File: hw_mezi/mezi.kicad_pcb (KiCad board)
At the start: 2 copper layers, 49.7 x 62.2 mm, 32 parts, among them J1 Conn_2Rows-05Pins, SW1 SW_DPST_x2, T1 Tab, T53,086 Tab, U1 PY32F002AF15P6TU

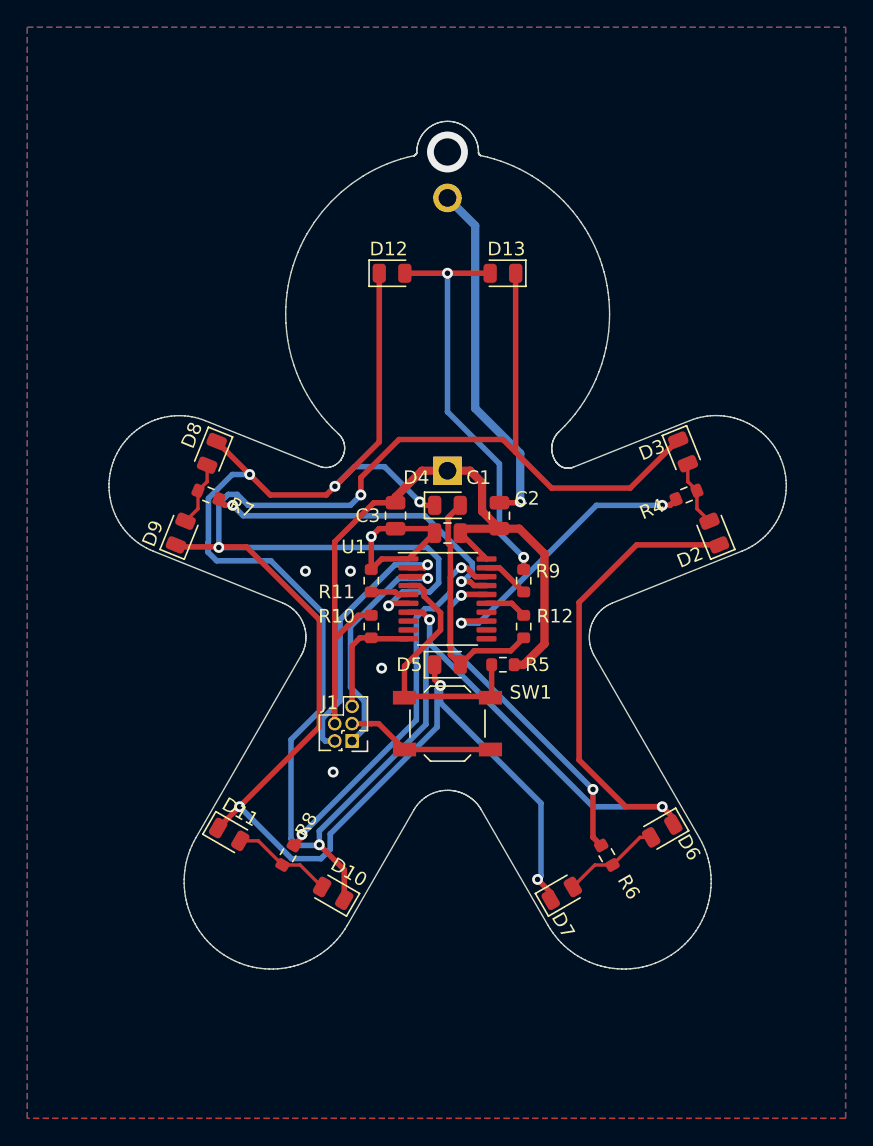
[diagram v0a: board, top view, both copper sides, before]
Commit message: mezi design update
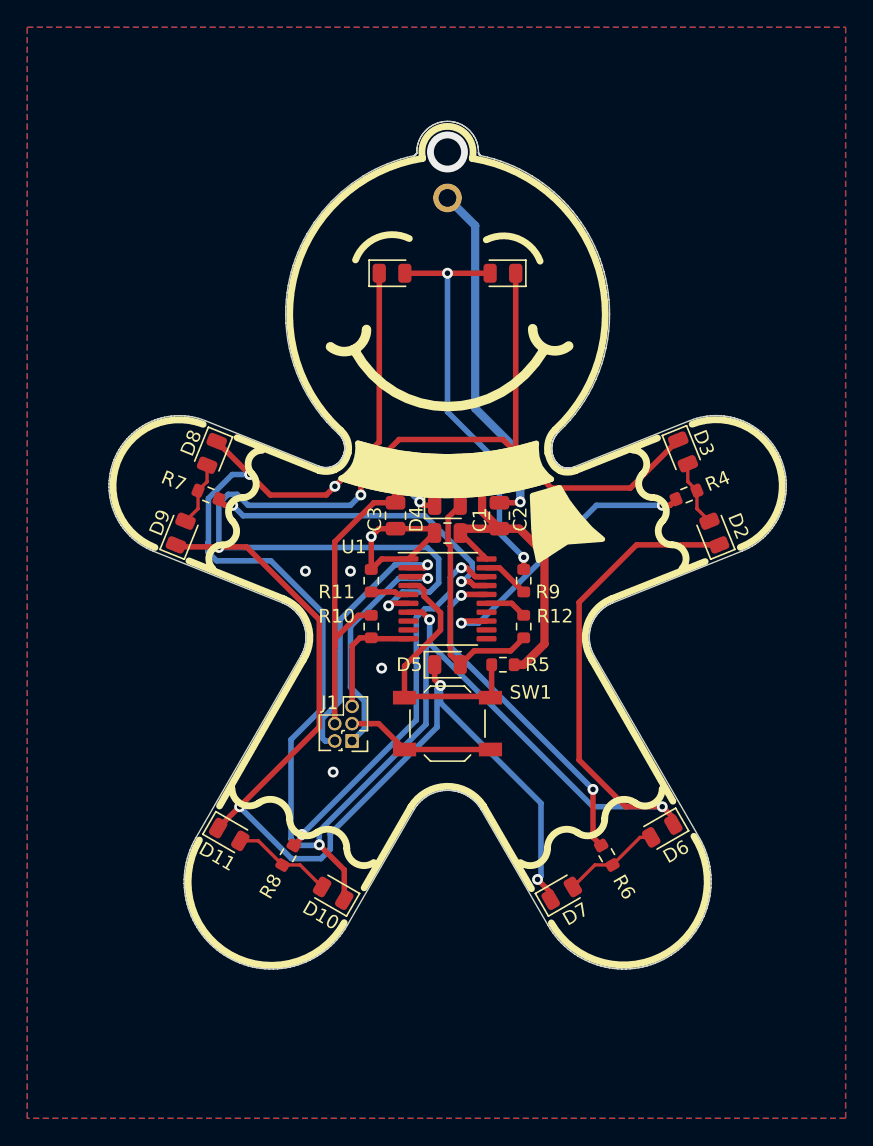
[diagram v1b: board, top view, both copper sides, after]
